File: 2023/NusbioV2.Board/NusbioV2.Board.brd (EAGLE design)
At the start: 88 x 77 mm, 27 parts

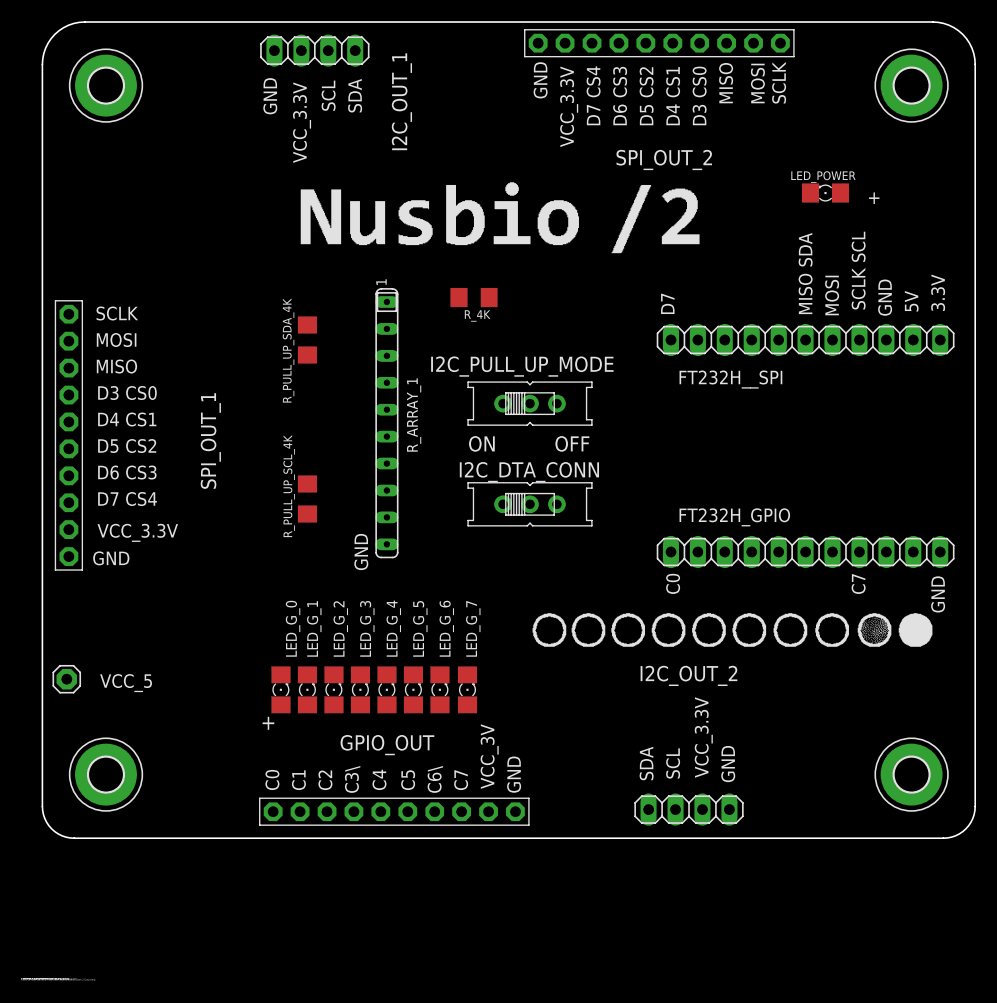
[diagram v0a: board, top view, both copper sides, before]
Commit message: Nsubio /2 v2 update
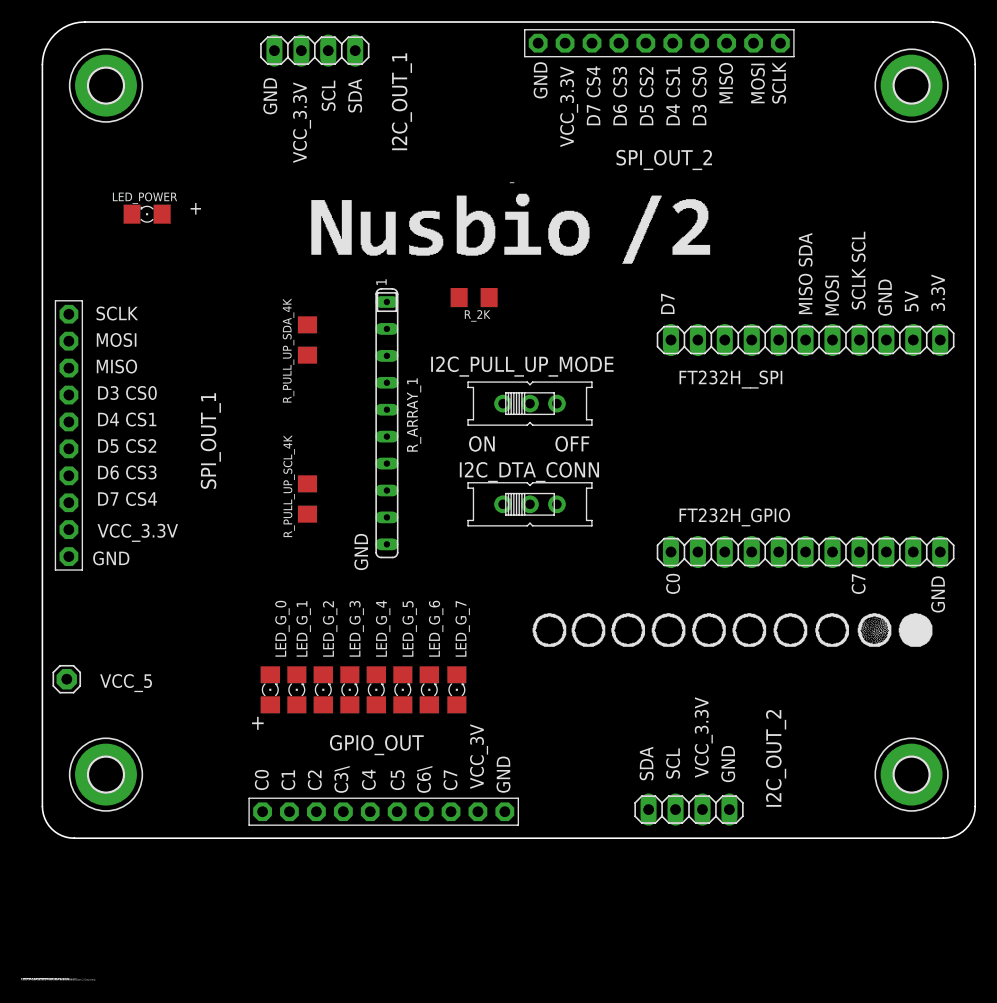
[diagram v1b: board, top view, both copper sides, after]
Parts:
- moved LED_POWER 64.0 mm to (11.9, 71.9)
- moved GPIO_OUT 1.00 mm to (34.2, 15.5)
- moved LED_G_0 1.00 mm to (23.5, 27.0)
- moved LED_G_1 1.00 mm to (26.0, 27.0)
- moved LED_G_2 1.00 mm to (28.5, 27.0)
- moved LED_G_3 1.00 mm to (31.0, 27.0)
- moved LED_G_4 1.00 mm to (33.5, 27.0)
- moved LED_G_5 1.00 mm to (36.0, 27.0)
- moved LED_G_6 1.00 mm to (38.5, 27.0)
- moved LED_G_7 1.00 mm to (41.1, 27.0)
- renumbered R_4K to R_2K
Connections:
- net VCC_33: now also LED_POWER.A
- net VCC_5: no longer LED_POWER.A

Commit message: Nsubio /2 v2 update
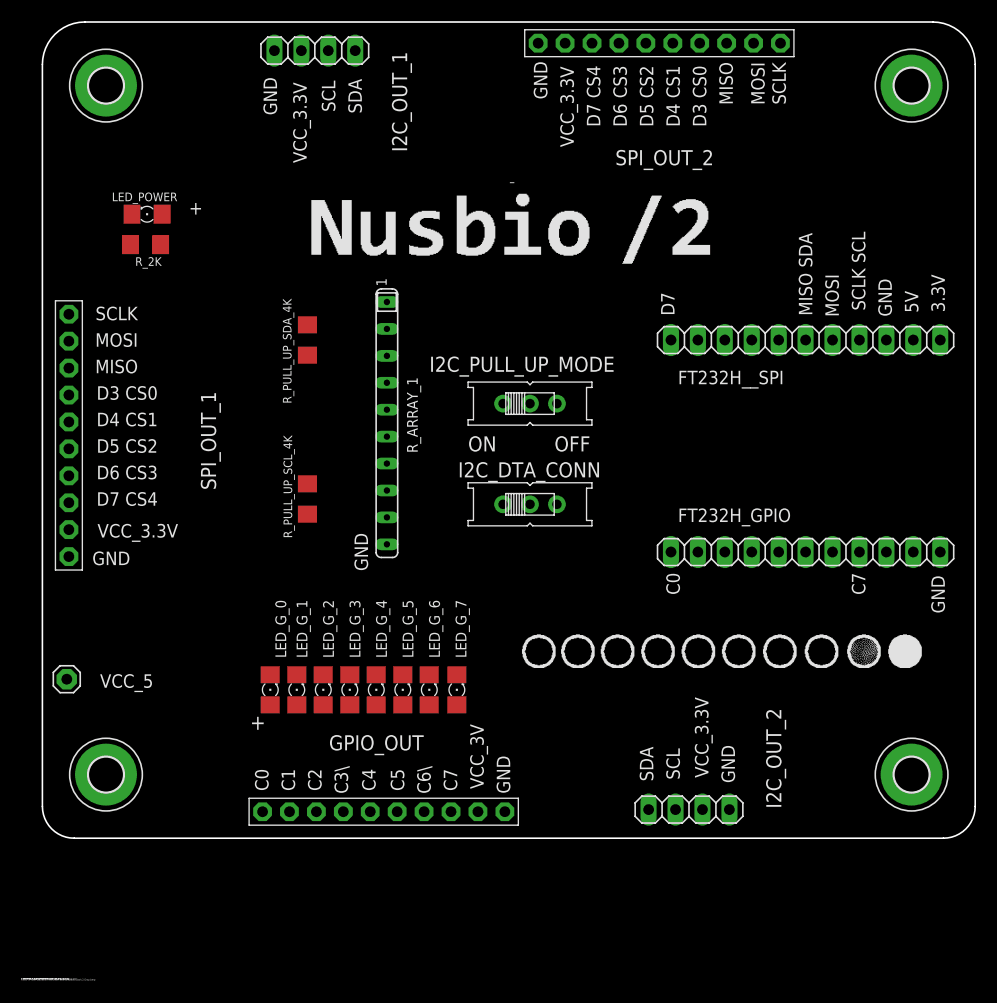
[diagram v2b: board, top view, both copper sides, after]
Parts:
- moved R_2K 31.4 mm to (11.7, 69.0)

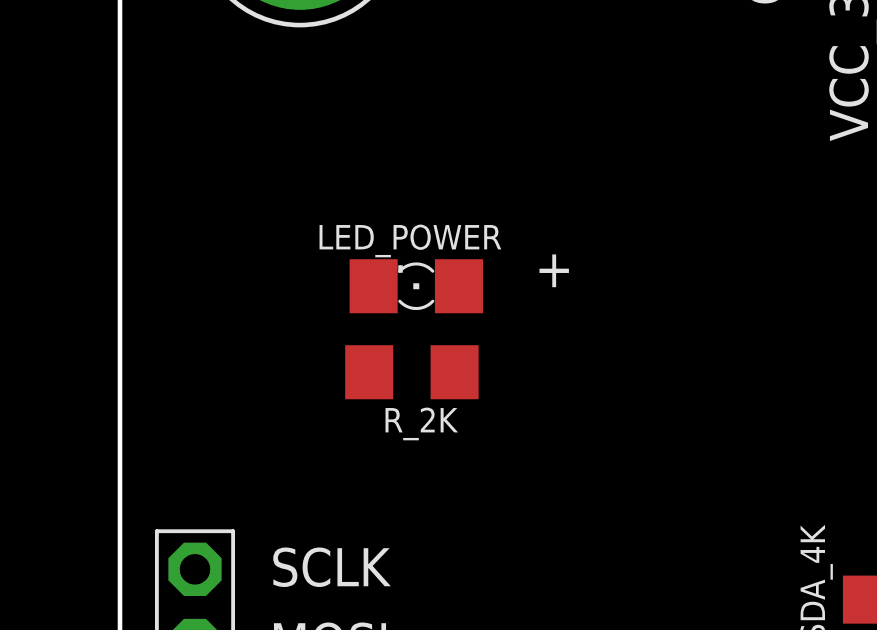
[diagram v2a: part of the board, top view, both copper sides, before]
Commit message: Nsubio /2 v2 update
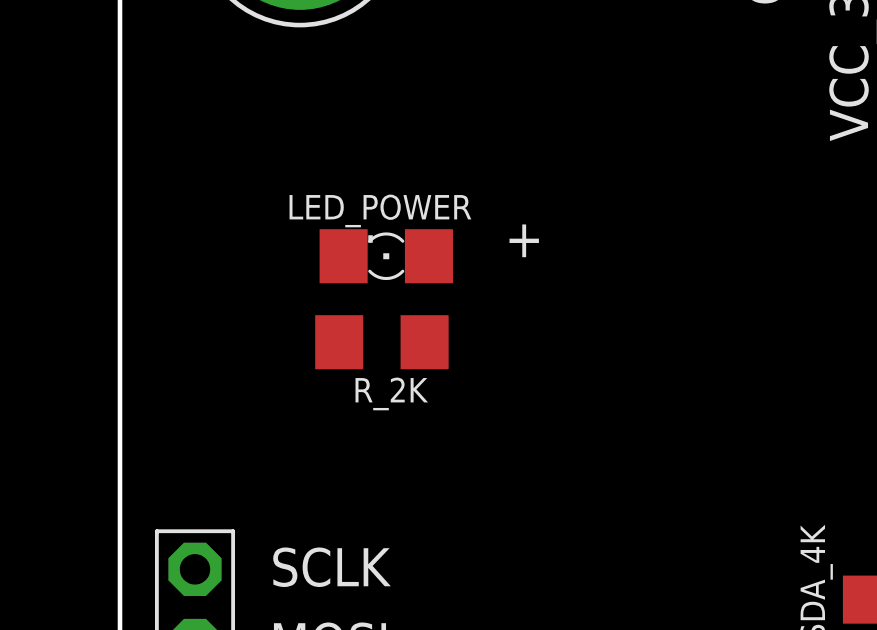
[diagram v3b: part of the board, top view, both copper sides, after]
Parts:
- moved LED_POWER 1.41 mm to (10.9, 72.9)
- moved R_2K 1.41 mm to (10.7, 70.0)
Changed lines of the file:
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@@
 <text x="46" y="28.5" size="2.54" layer="26" rot="SMR0" align="center">www.FredericTorres.com</text>
 <text x="86.5" y="36" size="1.27" layer="25" rot="R270" align="center">GND</text>
-<text x="16.47376875" y="72.468759375" size="1.27" layer="25" rot="R180" align="center">+</text>
+<text x="15.47376875" y="73.468759375" size="1.27" layer="25" rot="R180" align="center">+</text>
 <wire x1="2" y1="16" x2="2" y2="86" width="0.1524" layer="20"/>
 <wire x1="6" y1="90" x2="86" y2="90" width="0.1524" layer="20"/>
@@
 </autorouter>
 <elements>
-<element name="LED_POWER" library="adafruit" package="1206" value="" x="11.876134375" y="71.86644375" smashed="yes" rot="R180">
-<attribute name="NAME" x="11.646134375" y="73.5" size="0.8128" layer="25" rot="R180" align="center"/>
-<attribute name="VALUE" x="13.146134375" y="74.40644375" size="1.27" layer="27" rot="R180"/>
-</element>
-<element name="R_2K" library="adafruit" package="R1206" value="" x="11.73" y="69" smashed="yes" rot="R180">
-<attribute name="NAME" x="12" y="67.4" size="0.8128" layer="25" rot="R180" align="center"/>
-<attribute name="VALUE" x="13.127" y="71.413" size="1.27" layer="27" rot="R180"/>
+<element name="LED_POWER" library="adafruit" package="1206" value="" x="10.876134375" y="72.86644375" smashed="yes" rot="R180">
+<attribute name="NAME" x="10.646134375" y="74.5" size="0.8128" layer="25" rot="R180" align="center"/>
+<attribute name="VALUE" x="12.146134375" y="75.40644375" size="1.27" layer="27" rot="R180"/>
+</element>
+<element name="R_2K" library="adafruit" package="R1206" value="" x="10.73" y="70" smashed="yes" rot="R180">
+<attribute name="NAME" x="11" y="68.4" size="0.8128" layer="25" rot="R180" align="center"/>
+<attribute name="VALUE" x="12.127" y="72.413" size="1.27" layer="27" rot="R180"/>
 </element>
 <element name="FT232H__SPI" library="pinhead" library_urn="urn:adsk.eagle:library:325" package="1X11" package3d_urn="urn:adsk.eagle:package:22410/2" value="" x="74" y="60" smashed="yes">
@@
 <wire x1="23.89" y1="87.3" x2="48.77" y2="88" width="0" layer="19" extent="1-1"/>
 <wire x1="8" y1="84" x2="23.89" y2="87.3" width="0" layer="19" extent="1-1"/>
-<wire x1="13.152" y1="69" x2="8" y2="84" width="0" layer="19" extent="1-1"/>
-<wire x1="34.5" y1="63.585" x2="13.152" y2="69" width="0" layer="19" extent="1-1"/>
-<wire x1="4.5" y1="39.57" x2="13.152" y2="69" width="0" layer="19" extent="1-1"/>
+<wire x1="12.152" y1="70" x2="8" y2="84" width="0" layer="19" extent="1-1"/>
+<wire x1="34.5" y1="63.585" x2="12.152" y2="70" width="0" layer="19" extent="1-1"/>
+<wire x1="4.5" y1="39.57" x2="12.152" y2="70" width="0" layer="19" extent="1-1"/>
 <wire x1="8" y1="19" x2="4.5" y2="39.57" width="0" layer="19" extent="1-1"/>
 </signal>
@@
 <wire x1="51.31" y1="88" x2="48" y2="54" width="0" layer="19" extent="1-1"/>
 <wire x1="26.43" y1="87.3" x2="51.31" y2="88" width="0" layer="19" extent="1-1"/>
-<wire x1="13.298134375" y1="71.86644375" x2="26.43" y2="87.3" width="0" layer="19" extent="1-1"/>
-<wire x1="4.5" y1="42.11" x2="13.298134375" y2="71.86644375" width="0" layer="19" extent="1-1"/>
+<wire x1="12.298134375" y1="72.86644375" x2="26.43" y2="87.3" width="0" layer="19" extent="1-1"/>
+<wire x1="4.5" y1="42.11" x2="12.298134375" y2="72.86644375" width="0" layer="19" extent="1-1"/>
 <wire x1="43.09" y1="15.5" x2="48" y2="54" width="0" layer="19" extent="1-1"/>
 <wire x1="64.27" y1="15.7" x2="43.09" y2="15.5" width="0" layer="19" extent="1-1"/>
@@
 <contactref element="LED_POWER" pad="C"/>
 <contactref element="R_2K" pad="2"/>
-<wire x1="10.308" y1="69" x2="10.454134375" y2="71.86644375" width="0" layer="19" extent="1-1"/>
+<wire x1="9.308" y1="70" x2="9.454134375" y2="72.86644375" width="0" layer="19" extent="1-1"/>
 </signal>
 <signal name="VCC_5">
